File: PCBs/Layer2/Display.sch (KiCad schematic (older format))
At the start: 30 parts, among them J1 Conn_01x12_Male, SW1 SW_Push, SW2 SW_Push, SW3 SW_Push, SW4 SW_Push, SW5 SW_Push, SW6 SW_Push, U2 arduinomini

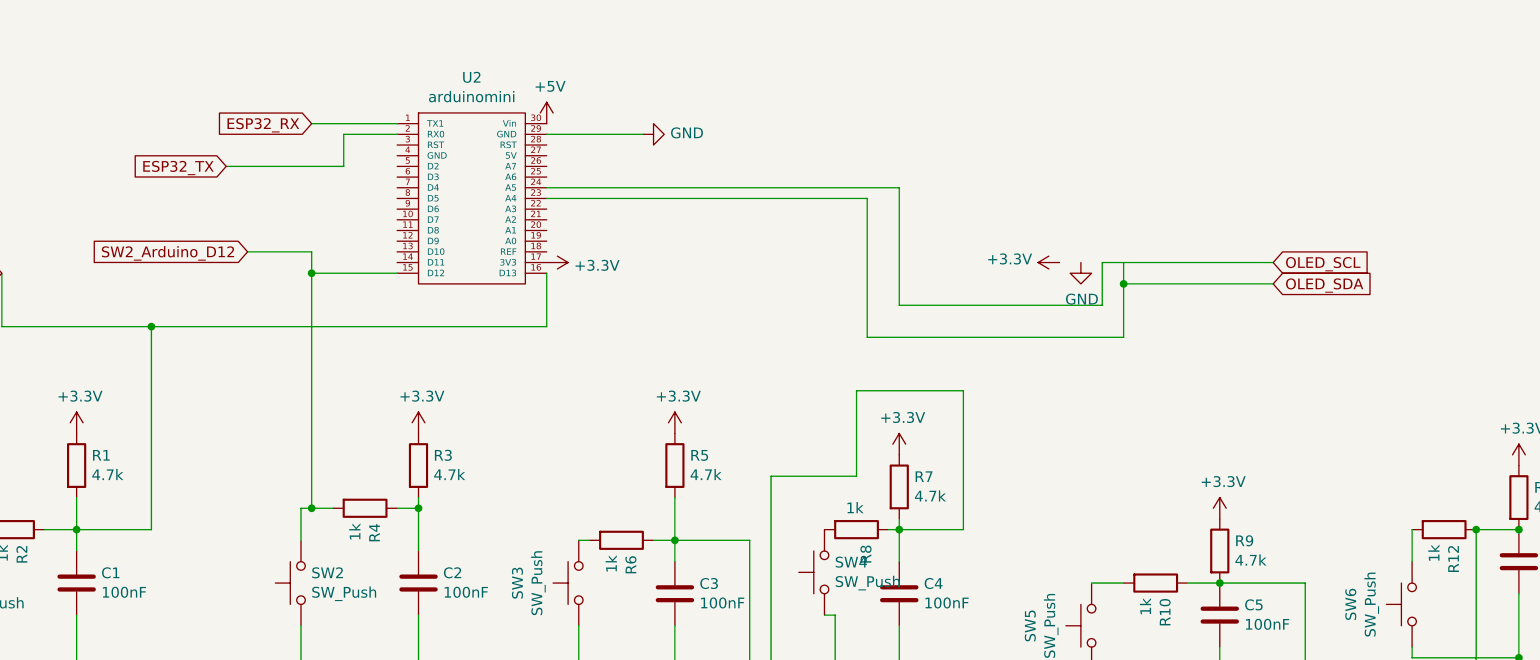
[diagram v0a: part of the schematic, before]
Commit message: display update
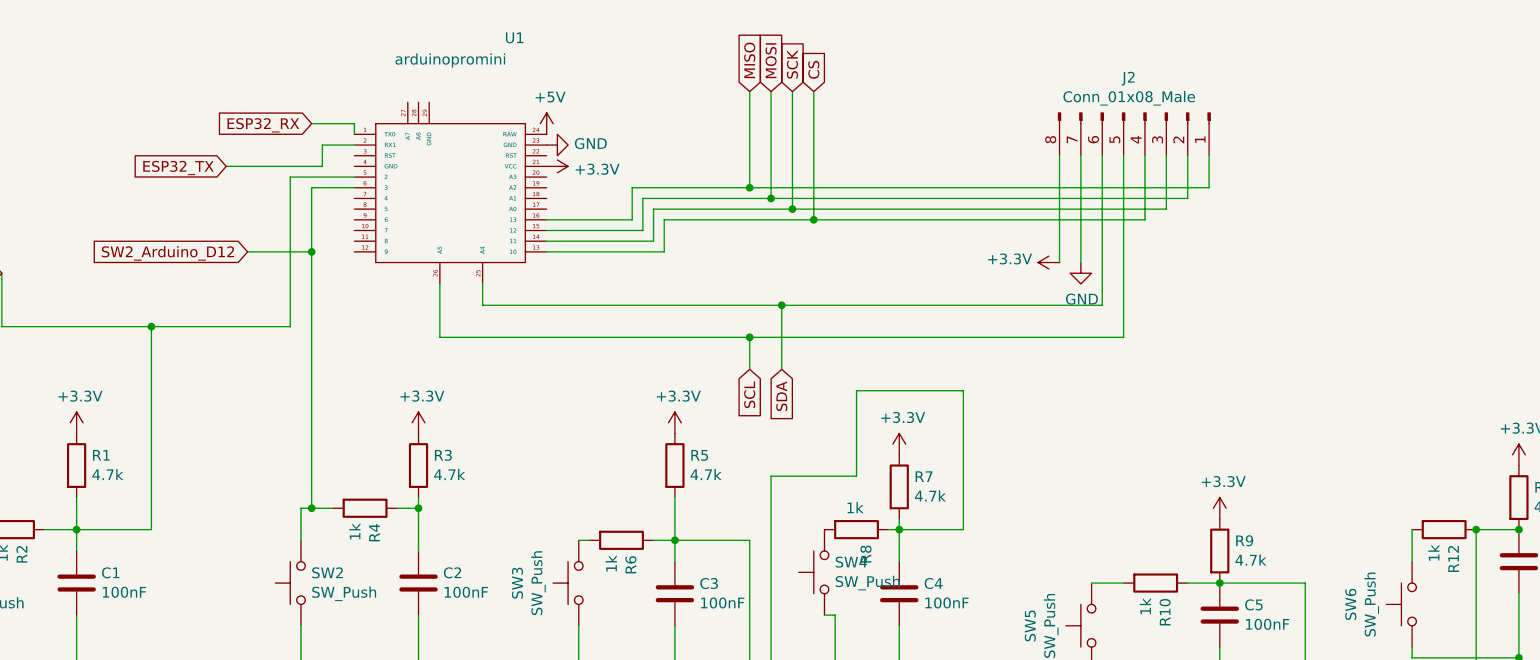
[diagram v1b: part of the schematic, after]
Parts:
- removed U2: arduinomini, Arduino_mini:Arduinomini, symbol arduinomini:arduinomini
- added J2: Conn_01x08_Male, Connector_PinHeader_2.54mm:PinHeader_1x08_P2.54mm_Vertical, symbol Connector:Conn_01x08_Male
- added U1: arduinopromini, arduinopromini:arduinopromini, symbol arduinopromini:arduinopromini
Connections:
- net +3V3: now also J2.8 (Pin_8), U1.21 (VCC)
- net +5V: now also U1.24 (RAW)
- net ESP32_RX: now also U1.1 (TX0)
- net ESP32_TX: now also U1.2 (RX1)
- net GND: now also J2.7 (Pin_7), U1.23 (GND)
- net SW1_Arduino_D13: now also U1.5 (2)
- net SW2_Arduino_D12: now also U1.6 (3)
- new net CS: J2.4 (Pin_4), U1.13 (10)
- new net MISO: J2.1 (Pin_1), U1.16 (13)
- new net MOSI: J2.2 (Pin_2), U1.15 (12)
- new net SCK: J2.3 (Pin_3), U1.14 (11)
- new net SCL: J2.5 (Pin_5), U1.26 (A5)
- new net SDA: J2.6 (Pin_6), U1.25 (A4)
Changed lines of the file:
@@
 Connection ~ 9750 3600
-$Comp
-L arduinomini:arduinomini U2
-U 1 1 5C6BE8D0
-P 4850 1450
-F 0 "U2" H 4850 2015 50  0000 C CNN
-F 1 "arduinomini" H 4850 1924 50  0000 C CNN
-F 2 "Arduino_mini:Arduinomini" H 4850 1950 50  0001 C CNN
-F 3 "" H 4850 1950 50  0001 C CNN
-	1    4850 1450
-	1    0    0    -1
-$EndComp
-Wire Wire Line
-	5200 1800 5200 2050
-Wire Wire Line
-	4500 1800 4100 1800
-Wire Wire Line
-	4100 1800 4100 2900
-Wire Wire Line
-	5200 1450 6700 1450
-Wire Wire Line
-	6700 1450 6700 2100
-Wire Wire Line
-	6700 2100 7900 2100
-Wire Wire Line
-	7900 2100 7900 1850
-Wire Wire Line
-	5200 1400 6850 1400
-Wire Wire Line
-	6850 1400 6850 1950
-Wire Wire Line
-	6850 1950 7800 1950
-Wire Wire Line
-	7800 1950 7800 1750
 $Comp
 L power:+3.3V #PWR021
@@
 Text GLabel 4100 1100 0    50   Input ~ 0
 ESP32_RX
-Wire Wire Line
-	4100 1100 4500 1100
 Text GLabel 3700 1300 0    50   Input ~ 0
 ESP32_TX
-Wire Wire Line
-	3700 1300 4250 1300
-Wire Wire Line
-	4250 1300 4250 1150
-Wire Wire Line
-	4250 1150 4500 1150
 $Comp
 L power:+5V #PWR016
 U 1 1 5C6C2935
-P 5200 1100
-F 0 "#PWR016" H 5200 950 50  0001 C CNN
-F 1 "+5V" H 5215 1273 50  0000 C CNN
-F 2 "" H 5200 1100 50  0001 C CNN
-F 3 "" H 5200 1100 50  0001 C CNN
-	1    5200 1100
+P 5200 1150
+F 0 "#PWR016" H 5200 1000 50  0001 C CNN
+F 1 "+5V" H 5215 1323 50  0000 C CNN
+F 2 "" H 5200 1150 50  0001 C CNN
+F 3 "" H 5200 1150 50  0001 C CNN
+	1    5200 1150
 	1    0    0    -1
 $EndComp
@@
 L power:GND #PWR019
 U 1 1 5C6C2992
-P 5650 1150
-F 0 "#PWR019" H 5650 900 50  0001 C CNN
-F 1 "GND" V 5655 1022 50  0000 R CNN
-F 2 "" H 5650 1150 50  0001 C CNN
-F 3 "" H 5650 1150 50  0001 C CNN
-	1    5650 1150
+P 5200 1200
+F 0 "#PWR019" H 5200 950 50  0001 C CNN
+F 1 "GND" V 5205 1072 50  0000 R CNN
+F 2 "" H 5200 1200 50  0001 C CNN
+F 3 "" H 5200 1200 50  0001 C CNN
+	1    5200 1200
 	0    -1   -1   0
 $EndComp
-Wire Wire Line
-	5200 1150 5650 1150
 Text GLabel 5750 5700 1    50   Input ~ 0
 ESP32_RX
@@
 L power:+3.3V #PWR017
 U 1 1 5C6D164A
-P 5200 1750
-F 0 "#PWR017" H 5200 1600 50  0001 C CNN
-F 1 "+3.3V" V 5215 1878 50  0000 L CNN
-F 2 "" H 5200 1750 50  0001 C CNN
-F 3 "" H 5200 1750 50  0001 C CNN
-	1    5200 1750
+P 5200 1300
+F 0 "#PWR017" H 5200 1150 50  0001 C CNN
+F 1 "+3.3V" V 5215 1428 50  0000 L CNN
+F 2 "" H 5200 1300 50  0001 C CNN
+F 3 "" H 5200 1300 50  0001 C CNN
+	1    5200 1300
 	0    1    1    0
 $EndComp
-Text GLabel 8600 1750 2    50   Input ~ 0
-OLED_SCL
-Wire Wire Line
-	7800 1750 8600 1750
-Text GLabel 8600 1850 2    50   Input ~ 0
-OLED_SDA
-Wire Wire Line
-	8600 1850 7900 1850
-Connection ~ 7900 1850
-Wire Wire Line
-	7900 1850 7900 1750
 Text GLabel 2650 1800 0    50   Input ~ 0
 SW1_Arduino_D13
@@
 	3800 1700 4100 1700
 Wire Wire Line
-	4100 1700 4100 1800
-Connection ~ 4100 1800
-Wire Wire Line
 	3350 2050 3350 3000
 Wire Wire Line
 	3350 3000 3000 3000
-Connection ~ 3350 2050
-Wire Wire Line
-	3350 2050 5200 2050
 Wire Wire Line
 	4600 2850 4600 2900
@@
 Wire Wire Line
 	9750 3300 9750 3600
+Wire Wire Line
+	7600 1750 7600 1250
+Wire Wire Line
+	7700 1750 7700 1250
+Wire Wire Line
+	7800 1250 7800 1950
+Wire Wire Line
+	7900 1250 7900 2100
+$Comp
+L arduinopromini:arduinopromini U1
+U 1 1 5C9155A1
+P 4750 1600
+F 0 "U1" H 5050 2500 50  0000 C CNN
+F 1 "arduinopromini" H 4750 2400 50  0000 C CNN
+F 2 "arduinopromini:arduinopromini" H 4750 2150 50  0001 C CNN
+F 3 "" H 4750 2150 50  0001 C CNN
+	1    4750 1600
+	1    0    0    -1
+$EndComp
+Wire Wire Line
+	4100 1700 4100 2900
+Wire Wire Line
+	4100 1100 4300 1100
+Wire Wire Line
+	4300 1100 4300 1150
+Wire Wire Line
+	3700 1300 4150 1300
+Wire Wire Line
+	4150 1300 4150 1200
+Wire Wire Line
+	4150 1200 4300 1200
+Wire Wire Line
+	3350 2050 4000 2050
+Wire Wire Line
+	4000 2050 4000 1350
+Wire Wire Line
+	4000 1350 4300 1350
+Connection ~ 3350 2050
+Wire Wire Line
+	4100 1700 4100 1400
+Wire Wire Line
+	4100 1400 4300 1400
+Connection ~ 4100 1700
+Wire Wire Line
+	4700 2100 4700 1850
+Wire Wire Line
+	4900 1950 4900 1850
+Text GLabel 6300 2250 3    50   Input ~ 0
+SDA
+Text GLabel 6150 2250 3    50   Input ~ 0
+SCL
+$Comp
+L Connector:Conn_01x08_Male J2
+U 1 1 5C94096F
+P 8000 1050
+F 0 "J2" V 7835 976 50  0000 C CNN
+F 1 "Conn_01x08_Male" V 7926 976 50  0000 C CNN
+F 2 "Connector_PinHeader_2.54mm:PinHeader_1x08_P2.54mm_Vertical" H 8000 1050 50  0001 C CNN
+F 3 "~" H 8000 1050 50  0001 C CNN
+	1    8000 1050
+	0    1    1    0
+$EndComp
+Wire Wire Line
+	5200 1650 5700 1650
+Wire Wire Line
+	5700 1650 5700 1500
+Wire Wire Line
+	5700 1500 6350 1500
+Wire Wire Line
+	8100 1500 8100 1250
+Wire Wire Line
+	5200 1600 5650 1600
+Wire Wire Line
+	5650 1600 5650 1450
+Wire Wire Line
+	5650 1450 6250 1450
+Wire Wire Line
+	8200 1450 8200 1250
+Wire Wire Line
+	5200 1550 5600 1550
+Wire Wire Line
+	5600 1550 5600 1400
+Wire Wire Line
+	5600 1400 6150 1400
+Wire Wire Line
+	8300 1400 8300 1250
+Wire Wire Line
+	4900 1950 6300 1950
+Wire Wire Line
+	4700 2100 6150 2100
+Wire Wire Line
+	5200 1700 5750 1700
+Wire Wire Line
+	5750 1700 5750 1550
+Wire Wire Line
+	5750 1550 6450 1550
+Wire Wire Line
+	8000 1550 8000 1250
+Wire Wire Line
+	6300 2250 6300 1950
+Connection ~ 6300 1950
+Wire Wire Line
+	6300 1950 7800 1950
+Wire Wire Line
+	6150 2250 6150 2100
+Connection ~ 6150 2100
+Wire Wire Line
+	6150 2100 7900 2100
+Text GLabel 6150 950  1    50   Input ~ 0
+MISO
+Text GLabel 6250 950  1    50   Input ~ 0
+MOSI
+Text GLabel 6350 950  1    50   Input ~ 0
+SCK
+Text GLabel 6450 950  1    50   Input ~ 0
+CS
+Wire Wire Line
+	6150 950  6150 1400
+Connection ~ 6150 1400
+Wire Wire Line
+	6150 1400 8300 1400
+Wire Wire Line
+	6250 950  6250 1450
+Connection ~ 6250 1450
+Wire Wire Line
+	6250 1450 8200 1450
+Wire Wire Line
+	6350 950  6350 1500
+Connection ~ 6350 1500
+Wire Wire Line
+	6350 1500 8100 1500
+Wire Wire Line
+	6450 950  6450 1550
+Connection ~ 6450 1550
+Wire Wire Line
+	6450 1550 8000 1550
 $EndSCHEMATC
